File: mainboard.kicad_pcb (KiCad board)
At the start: 2 copper layers, 81.3 x 73 mm, 63 parts, among them J1 Screw_Terminal_1x02, J2 SERVO 5V, Q1 IRLR024NPBF, U1 AT90CAN128-16MU, U2 MCP2551-I/SN, U3 EP_MODULE, Y1 Crystal

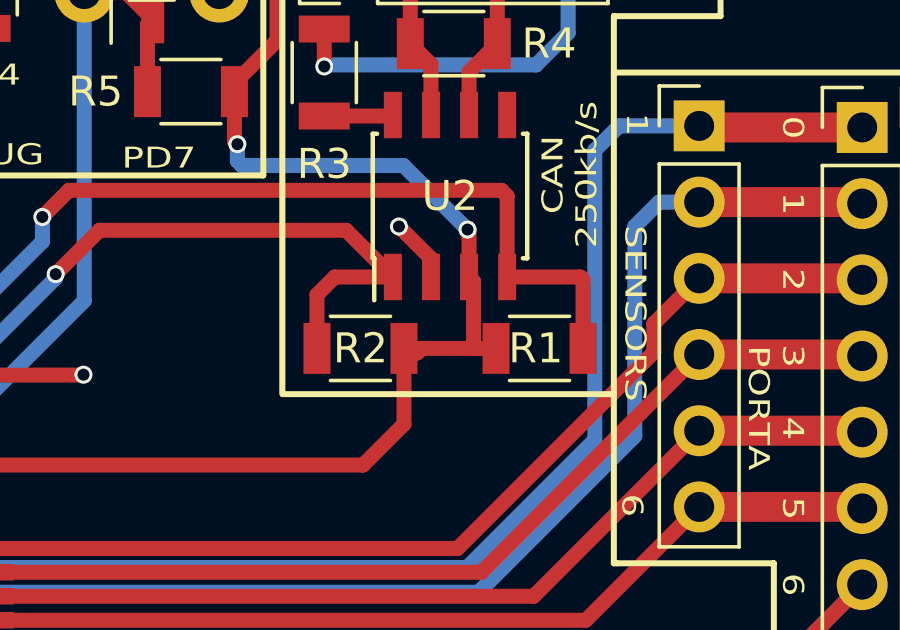
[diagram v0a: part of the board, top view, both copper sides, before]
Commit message: Small modif
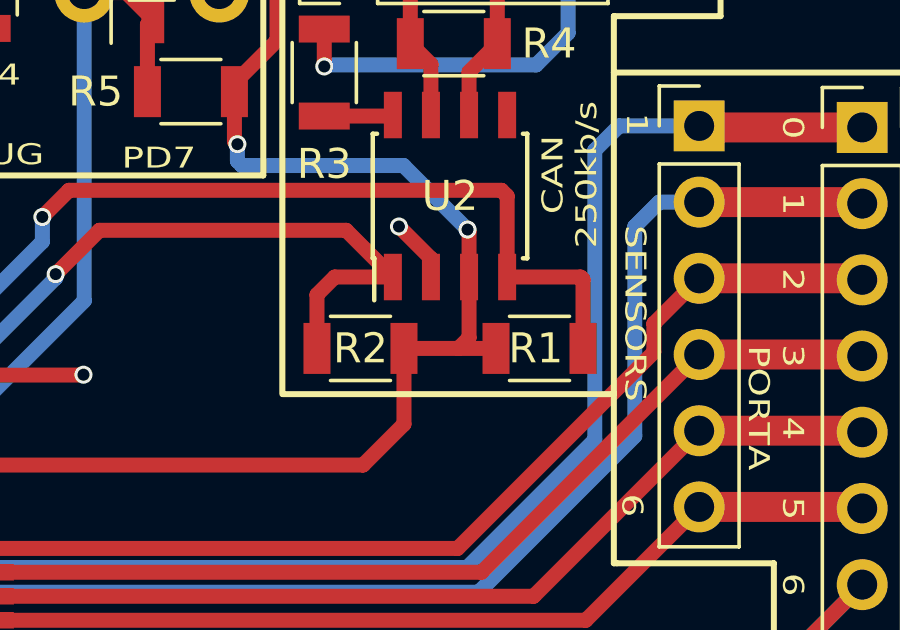
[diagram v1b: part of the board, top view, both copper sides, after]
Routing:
- net +5V: track 308.3 -> 307.7 mm
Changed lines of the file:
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@@
   (general
     (links 227)
-    (no_connects 7)
+    (no_connects 6)
     (area 62.154999 36.246999 143.585001 109.422001)
     (thickness 1.6)
-    (drawings 237)
-    (tracks 734)
+    (drawings 238)
+    (tracks 732)
     (zones 0)
     (modules 63)
@@
     (pad 1 thru_hole circle (at 0 0) (size 4.064 4.064) (drill 3.048) (layers *.Cu *.Mask F.SilkS))
   )
+  (gr_line (start 122.0216 92.1512) (end 120.3452 90.4748) (angle 90) (layer B.Paste) (width 0.2))
   (gr_line (start 108.331 57.277) (end 76.581 57.277) (angle 90) (layer B.Paste) (width 0.2))
   (gr_line (start 108.331 53.467) (end 108.331 57.277) (angle 90) (layer B.Paste) (width 0.2))
@@
   (gr_line (start 70.8025 86.487) (end 70.8025 106.934) (angle 90) (layer B.Paste) (width 0.2))
   (gr_line (start 62.738 86.487) (end 70.8025 86.487) (angle 90) (layer B.Paste) (width 0.2))
-  (gr_text PC (at 120.396 92.456) (layer B.Paste)
+  (gr_text PC (at 120.142 89.408) (layer B.Paste)
     (effects (font (size 1.5 1.5) (thickness 0.3)) (justify mirror))
   )
@@
   (segment (start 101.962 80.3465) (end 104.5465 82.931) (width 0.5) (layer F.Cu) (net 3))
   (segment (start 104.5465 82.931) (end 105.723 82.931) (width 0.5) (layer F.Cu) (net 3))
+  (segment (start 125.984 55.278) (end 125.984 57.3024) (width 0.5) (layer F.Cu) (net 4) (status 400000))
+  (segment (start 125.984 57.3024) (end 125.6284 57.658) (width 0.5) (layer F.Cu) (net 4))
+  (segment (start 123.8145 57.658) (end 125.6284 57.658) (width 0.5) (layer F.Cu) (net 4) (status 400000))
+  (segment (start 125.6284 57.658) (end 126.8835 57.658) (width 0.5) (layer F.Cu) (net 4) (status 800000))
   (segment (start 108.9152 61.5456) (end 122.452 61.5456) (width 0.5) (layer F.Cu) (net 4) (status 400000))
   (segment (start 123.8145 60.1831) (end 123.8145 57.658) (width 0.5) (layer F.Cu) (net 4) (status 800000))
   (segment (start 122.452 61.5456) (end 123.8145 60.1831) (width 0.5) (layer F.Cu) (net 4))
-  (segment (start 123.8145 57.658) (end 124.4092 57.658) (width 0.5) (layer F.Cu) (net 4))
-  (segment (start 126.8835 57.658) (end 124.4092 57.658) (width 0.5) (layer F.Cu) (net 4))
-  (segment (start 124.4092 57.658) (end 124.2568 57.8104) (width 0.5) (layer F.Cu) (net 4))
-  (segment (start 124.2568 57.8104) (end 123.8145 57.658) (width 0.5) (layer F.Cu) (net 4))
   (segment (start 99.562 78.82) (end 99.562 76.5242) (width 0.5) (layer F.Cu) (net 4))
   (segment (start 95.504 60.7441) (end 95.504 55.499) (width 0.5) (layer B.Cu) (net 4))
@@
   (segment (start 119.5832 45.5422) (end 120.2944 44.831) (width 0.5) (layer F.Cu) (net 4))
   (segment (start 120.2944 44.831) (end 121.666 44.831) (width 0.5) (layer F.Cu) (net 4))
-  (segment (start 126.1342 57.658) (end 126.1342 55.4282) (width 0.5) (layer F.Cu) (net 4))
-  (segment (start 126.1342 55.4282) (end 125.984 55.278) (width 0.5) (layer F.Cu) (net 4))
   (segment (start 95.274 61.087) (end 95.274 56.699) (width 0.5) (layer F.Cu) (net 4))
   (segment (start 95.274 56.699) (end 94.074 55.499) (width 0.5) (layer F.Cu) (net 4))
